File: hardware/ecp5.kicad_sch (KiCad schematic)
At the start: 8 parts, among them U3 ECP5U_12_CABGA256

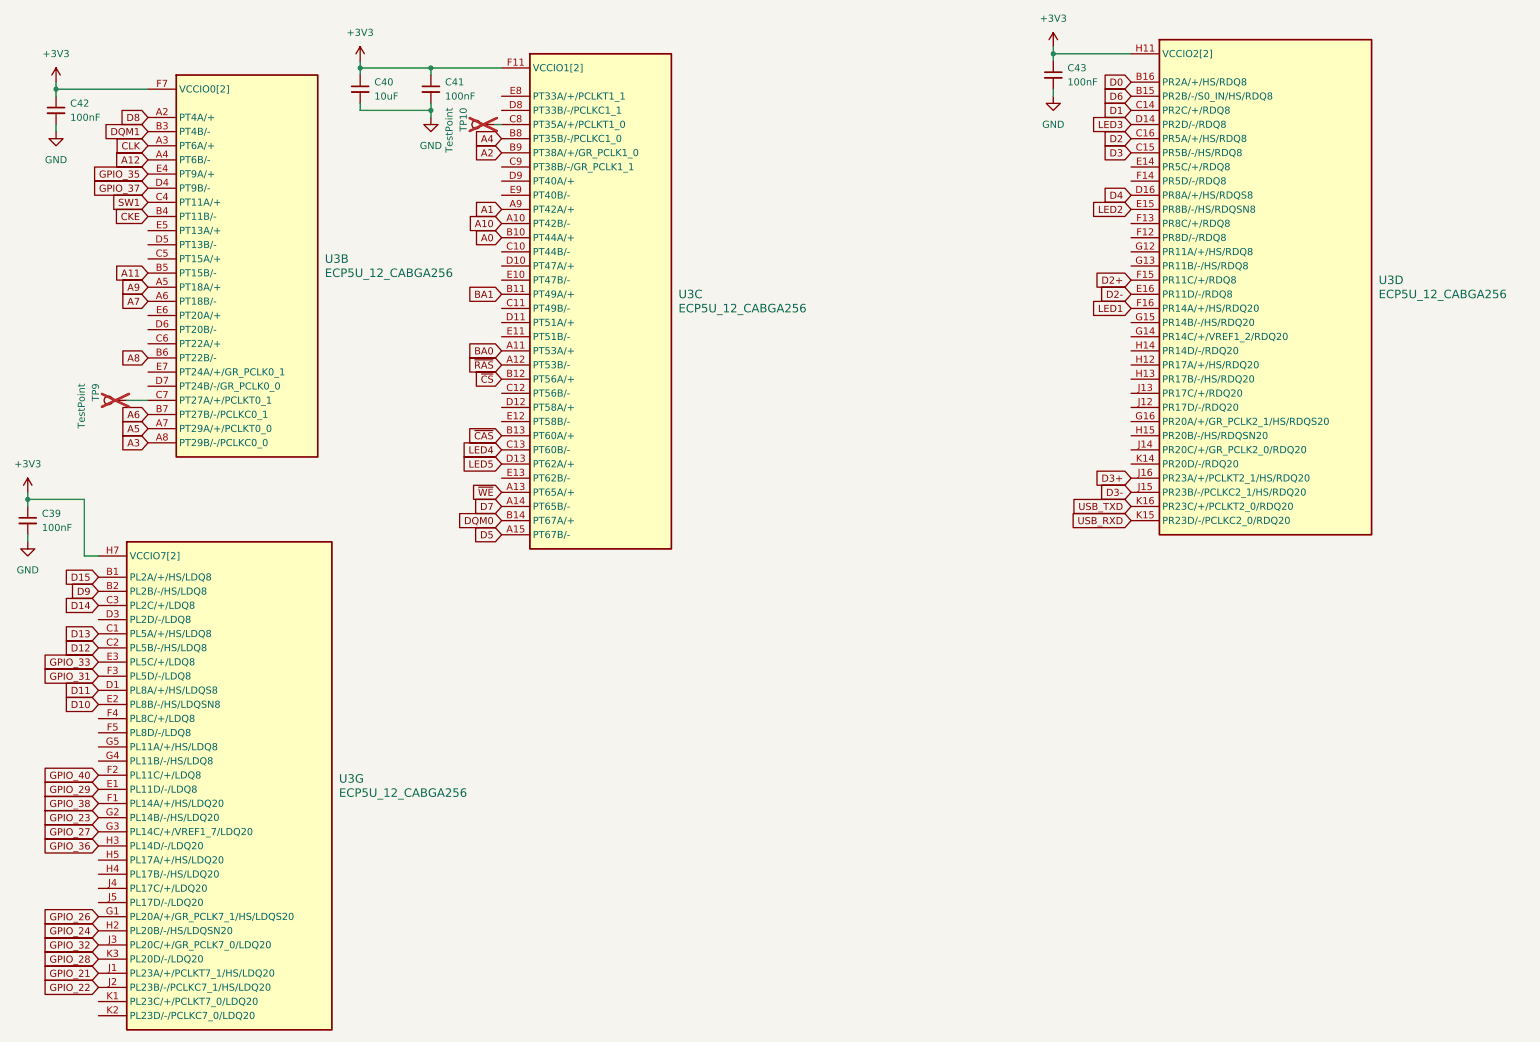
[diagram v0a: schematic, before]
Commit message: Final revision
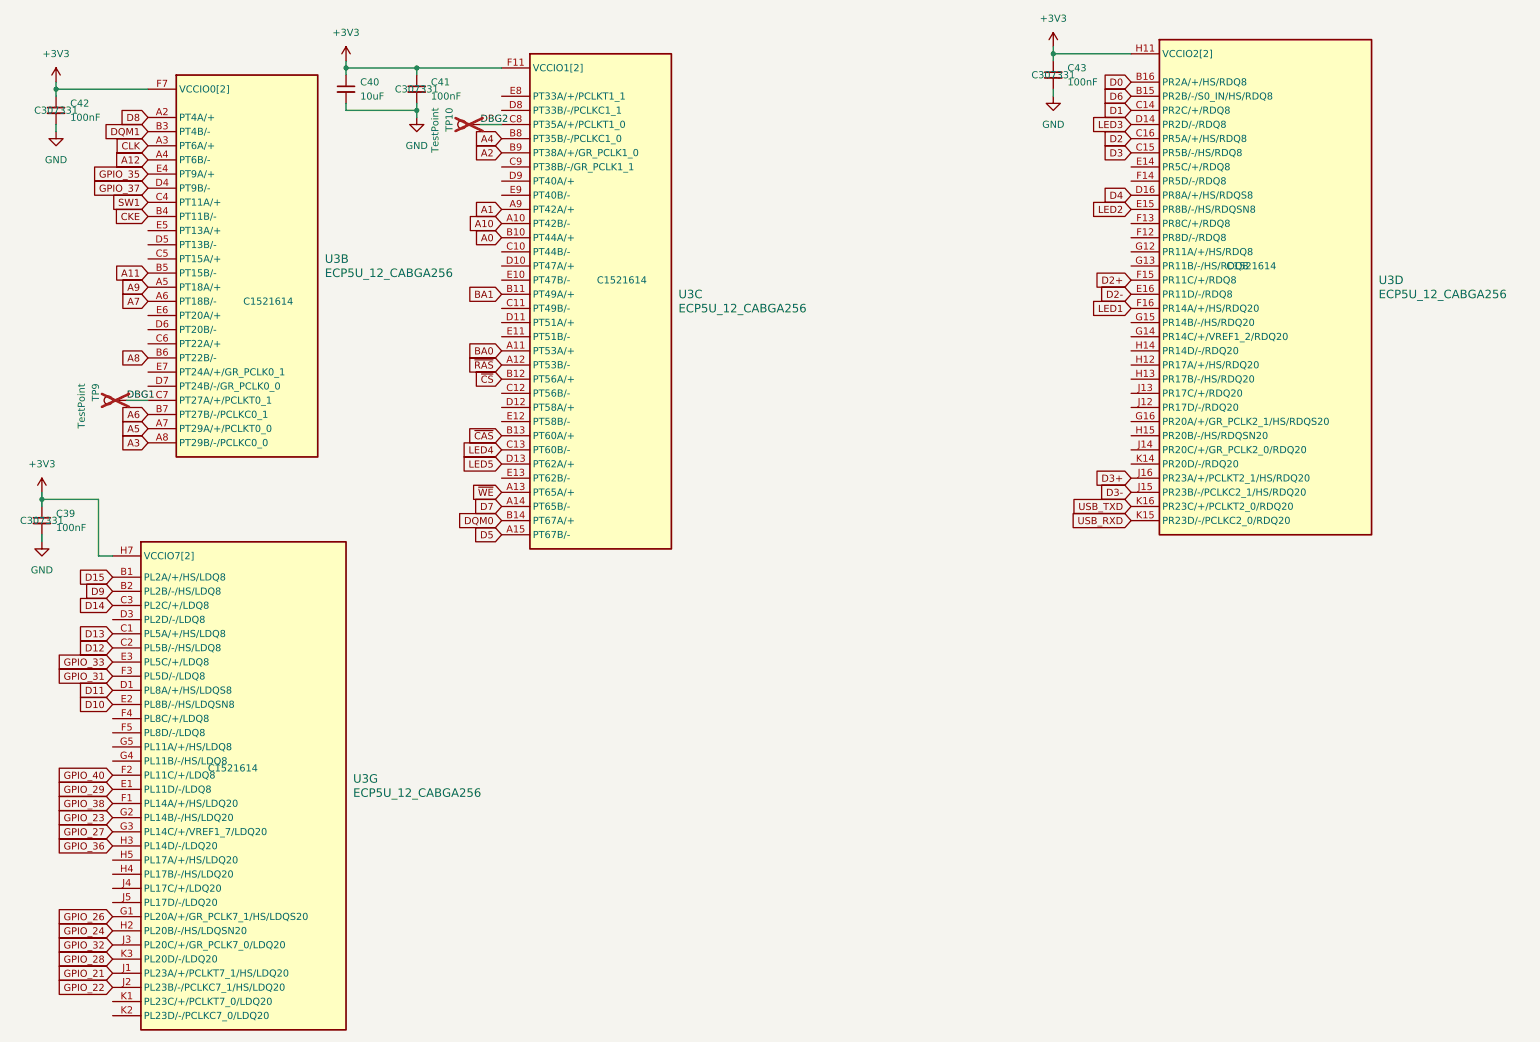
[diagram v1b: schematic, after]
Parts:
- C39, C41, C42, C43: JLCPCB Part # C307331 -> (none); LCSC Part # (none) -> C307331
- U3: JLCPCB Part # C1521614 -> (none); LCSC Part # (none) -> C1521614
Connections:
- net DBG1: now reaches TP9.1, U3.C7 (PT27A/+/PCLKT0_1)
- net DBG2: now reaches TP10.1, U3.C8 (PT35A/+/PCLKT1_0)
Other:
- moved on the sheet: C39, C40, C41, TP10, U3G

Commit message: Last checks
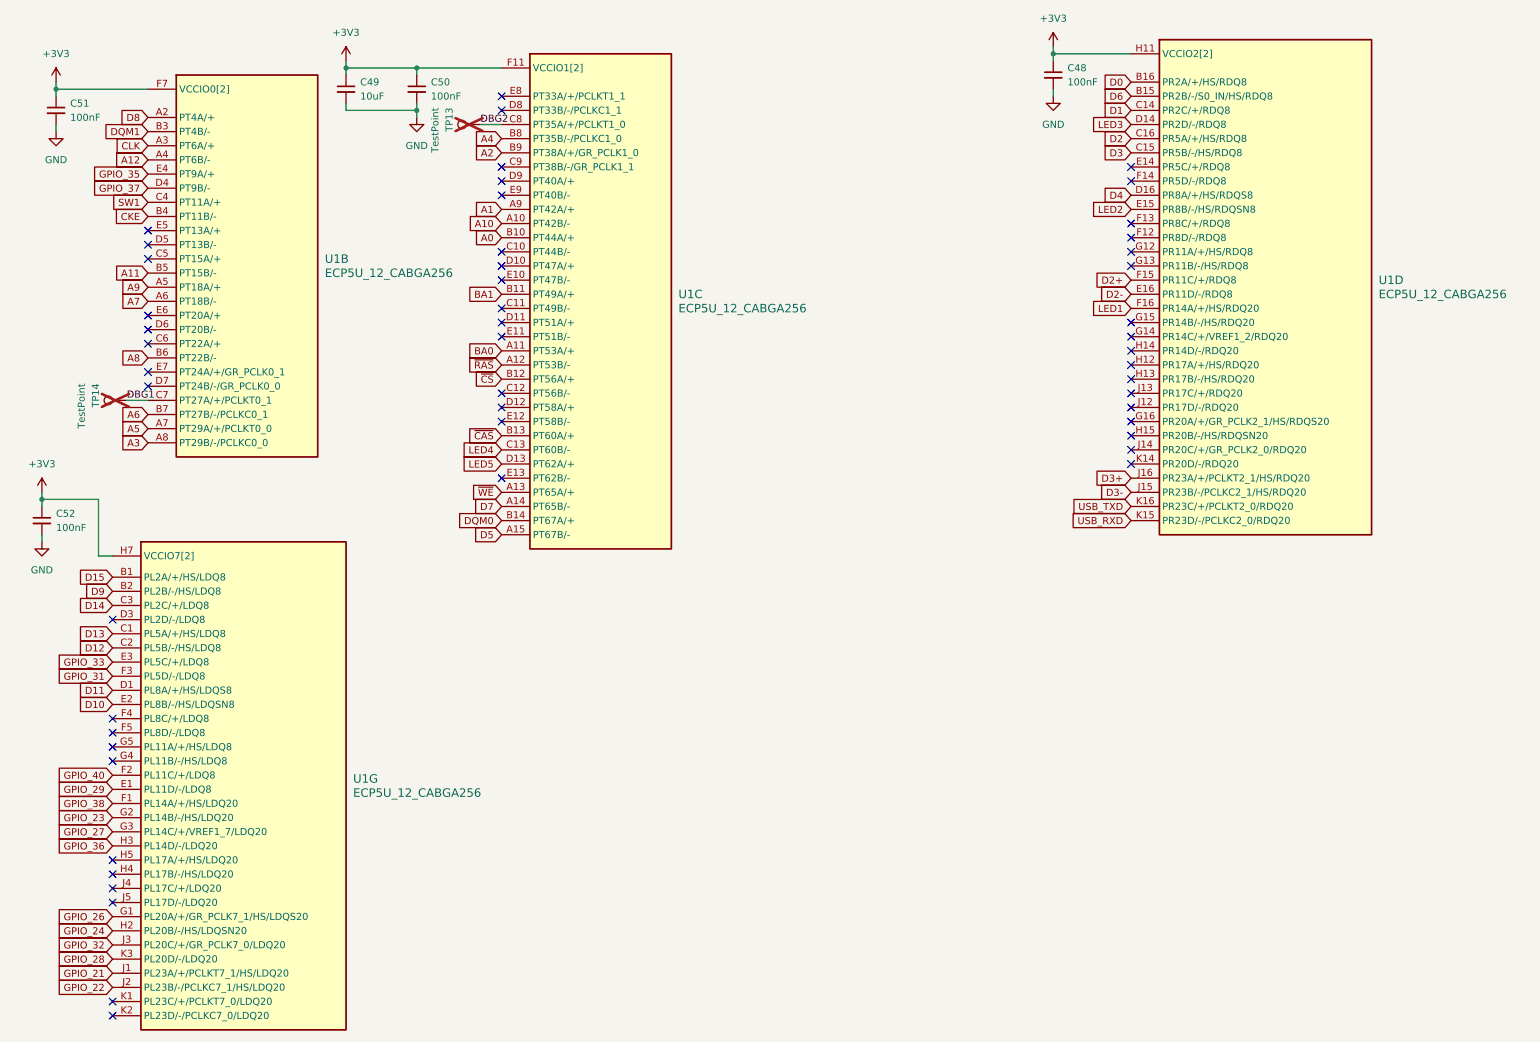
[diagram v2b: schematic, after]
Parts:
- C49: renamed from C40; LCSC Part # (none) -> C19702
- renumbered C43 to C48, C41 to C50, C42 to C51, C39 to C52, TP10 to TP13, TP9 to TP14, U3 to U1
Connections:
- no-connect marks 0 -> 51
